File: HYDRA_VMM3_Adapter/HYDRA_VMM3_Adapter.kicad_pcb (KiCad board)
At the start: 10 copper layers, 121.5 x 31.5 mm, 7 parts, among them J1 ME1014010101011, J2 ME1014010101011, J3 ME1014010101011, J4 ME1014010101011, J5 ME1014010101011, J6 ME1014010101011

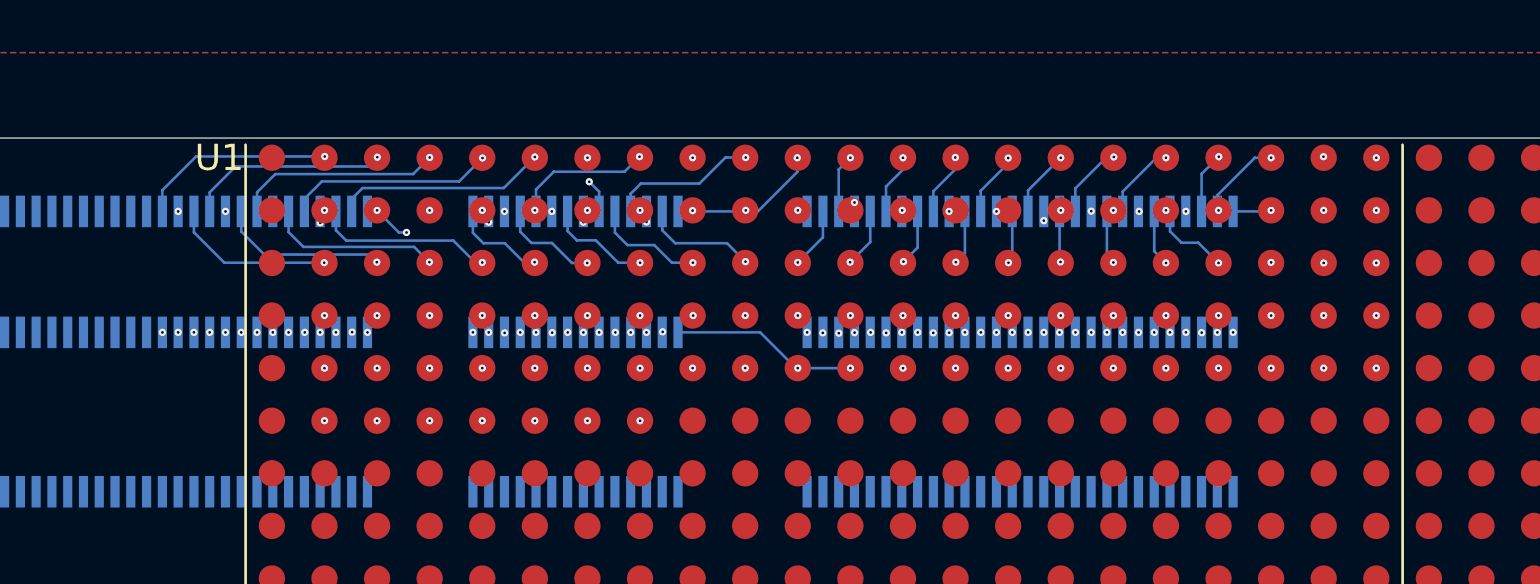
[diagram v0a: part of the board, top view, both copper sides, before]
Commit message: .
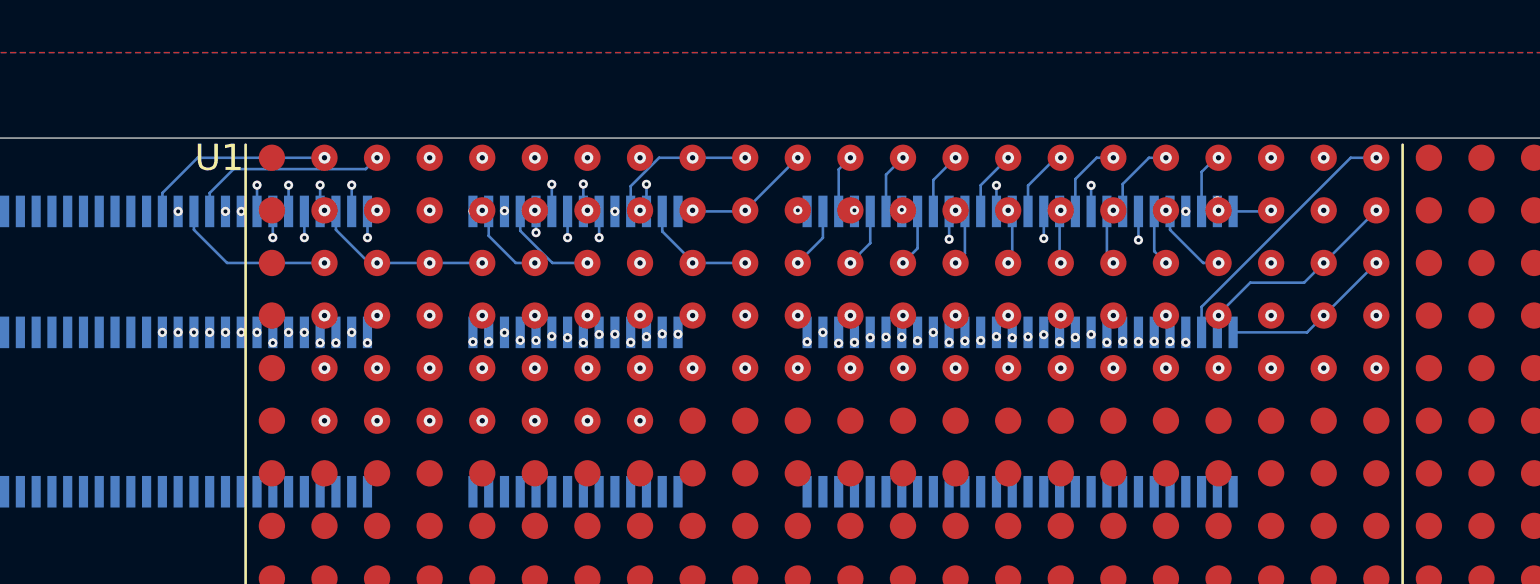
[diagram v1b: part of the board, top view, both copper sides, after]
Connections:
- J4 pad A59: Col_20-Row_4 -> Col_20-Row_3
- J4 pad A60: Col_20-Row_3 -> Col_20-Row_4
- J4 pad B29: Col_6-Row_3 -> Col_7-Row_1
- J4 pad B30: Col_7-Row_1 -> Col_6-Row_3
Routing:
- net Col_14-Row_2: track 0.62 -> 2.88 mm, vias 1 -> 2
- net Col_15-Row_2: track 0.46 -> 2.59 mm, vias 1 -> 2
- net Col_22-Row_1: track 11.6 -> 9.96 mm, vias 2 -> 1
- net Col_18-Row_2: track 1.06 -> 2.65 mm
- net Col_5-Row_2: track 6.35 -> 7.88 mm
- net Col_21-Row_1: track 12.5 -> 11.0 mm
- net Col_16-Row_2: track 1.16 -> 2.59 mm
- net Col_17-Row_2: track 0.90 -> 2.32 mm
- net Col_21-Row_2: track 10.4 -> 11.6 mm
- net Col_10-Row_2: track 3.98 -> 5.20 mm
- net Col_8-Row_2: track 4.08 -> 5.28 mm
- net Col_18-Row_4: track 7.05 -> 8.24 mm
- net Col_5-Row_1: track 7.91 -> 9.02 mm, vias 1 -> 2
- net Col_19-Row_4: track 7.51 -> 8.62 mm
- net Col_20-Row_3: track 8.67 -> 9.78 mm, vias 2 -> 3
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- removed copper zone on In7.Cu, net GND
- removed copper zone on In8.Cu, net GND
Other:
- copper layers 10 -> 8
